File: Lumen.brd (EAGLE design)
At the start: 59.3 x 24 mm, 33 parts, among them J1 AVR_SPI_PRG_6PTH, U1 Tiny45-20-SMT, Y1 8Mhz

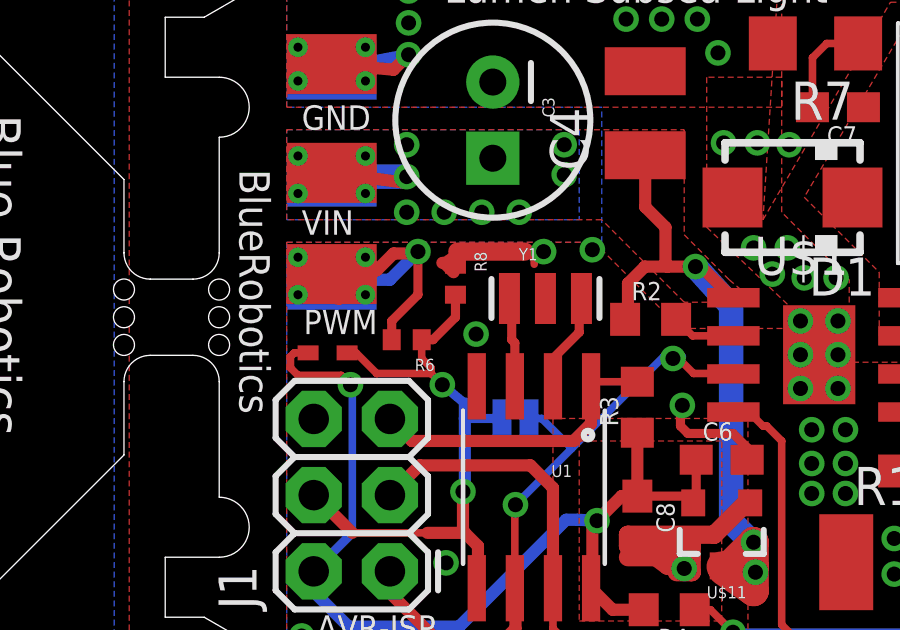
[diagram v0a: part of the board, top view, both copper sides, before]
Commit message: Minor layout updates for new production order.
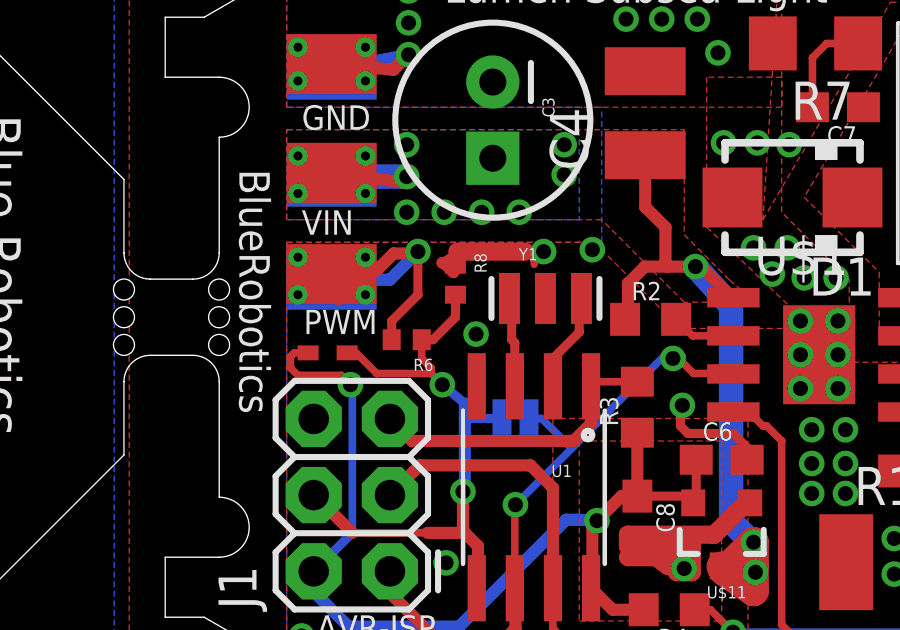
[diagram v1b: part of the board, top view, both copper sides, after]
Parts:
- R6, R8: device BlueRobotics-Main:C0402 -> BlueRobotics-Main:R0402
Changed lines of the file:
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@@
 <element name="C7" library="resistor" package="C0603" value="NP" x="46.625" y="19" rot="R180"/>
 <element name="R7" library="resistor" package="R1206" value="NP" x="45.875" y="21.125" rot="R180"/>
-<element name="R6" library="BlueRobotics-Main" package="C0402" value="15K 1/5W" x="32.25" y="11.25" rot="R180"/>
-<element name="R8" library="BlueRobotics-Main" package="C0402" value="300K" x="33.875" y="13.25" rot="R270"/>
+<element name="R6" library="BlueRobotics-Main" package="R0402" value="15K 1/5W" x="32.25" y="11.25" rot="R180"/>
+<element name="R8" library="BlueRobotics-Main" package="R0402" value="300K" x="33.875" y="13.25" rot="R270"/>
 <element name="Y1" library="SparkFun" package="RESONATOR-SMD" value="8Mhz" x="36.875" y="12.625"/>
 </elements>
